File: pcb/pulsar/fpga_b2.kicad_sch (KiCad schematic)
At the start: 85 parts

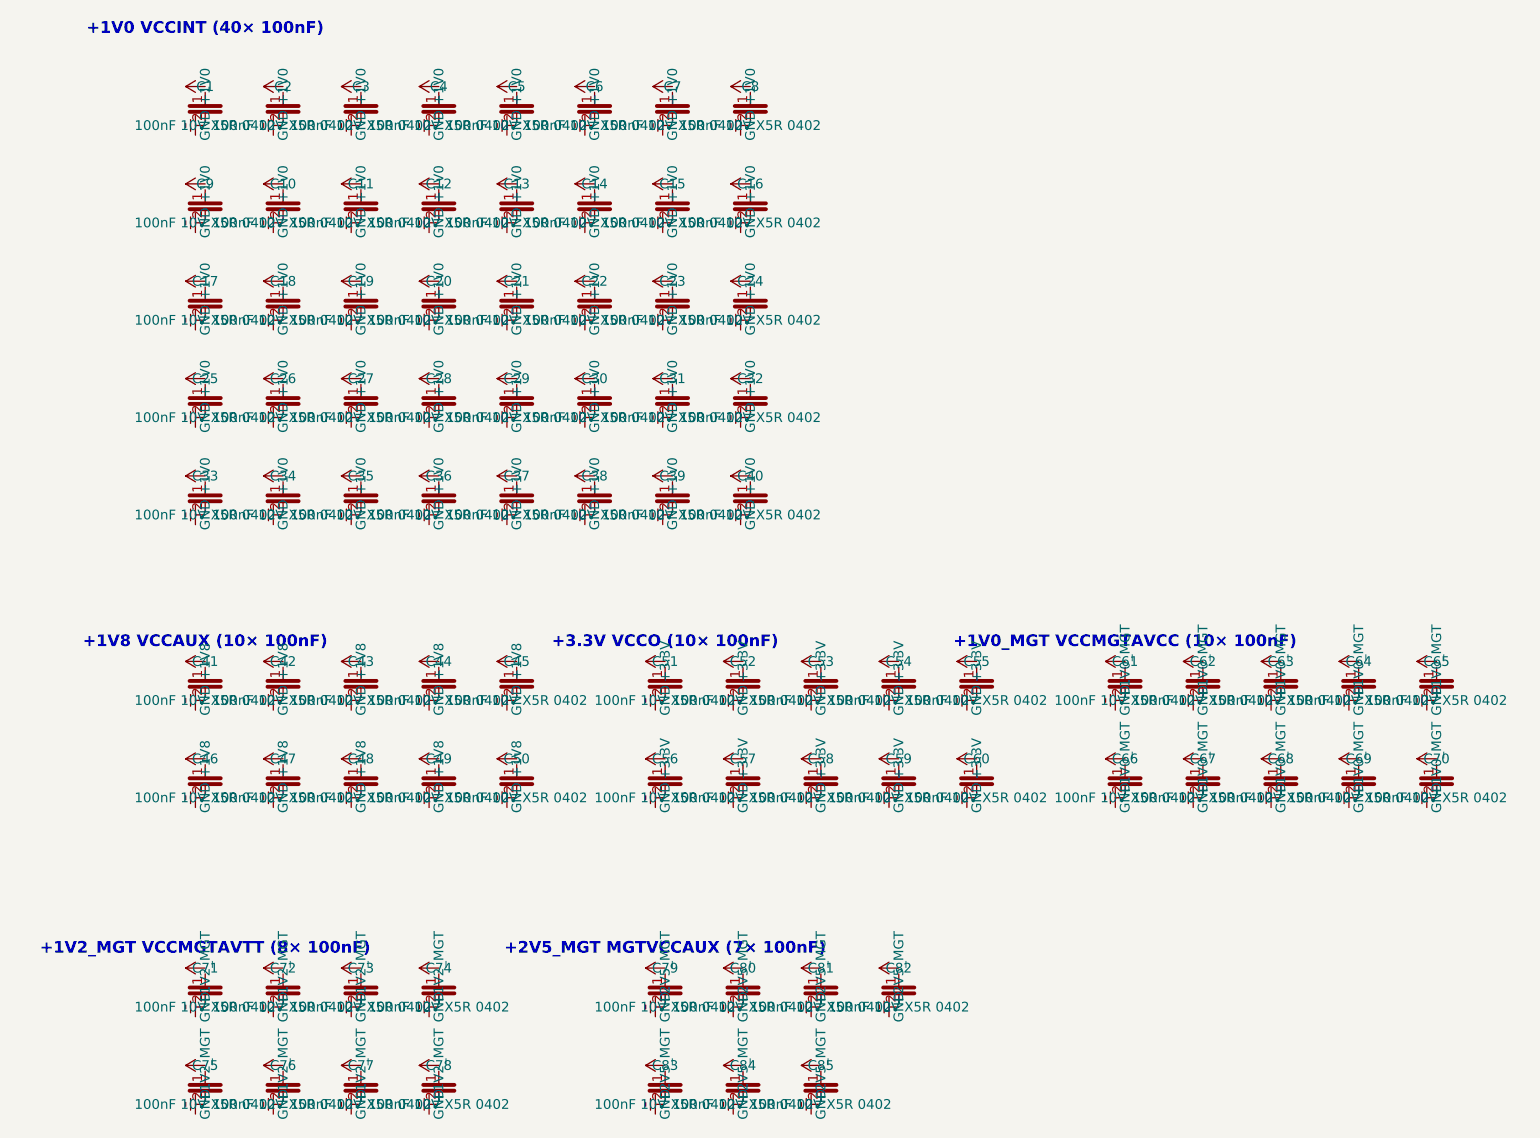
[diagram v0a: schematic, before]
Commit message: feat: let everything to route
Signed-off-by: Axel Ibarrondo <135344010+Axel84727@users.noreply.github.com>
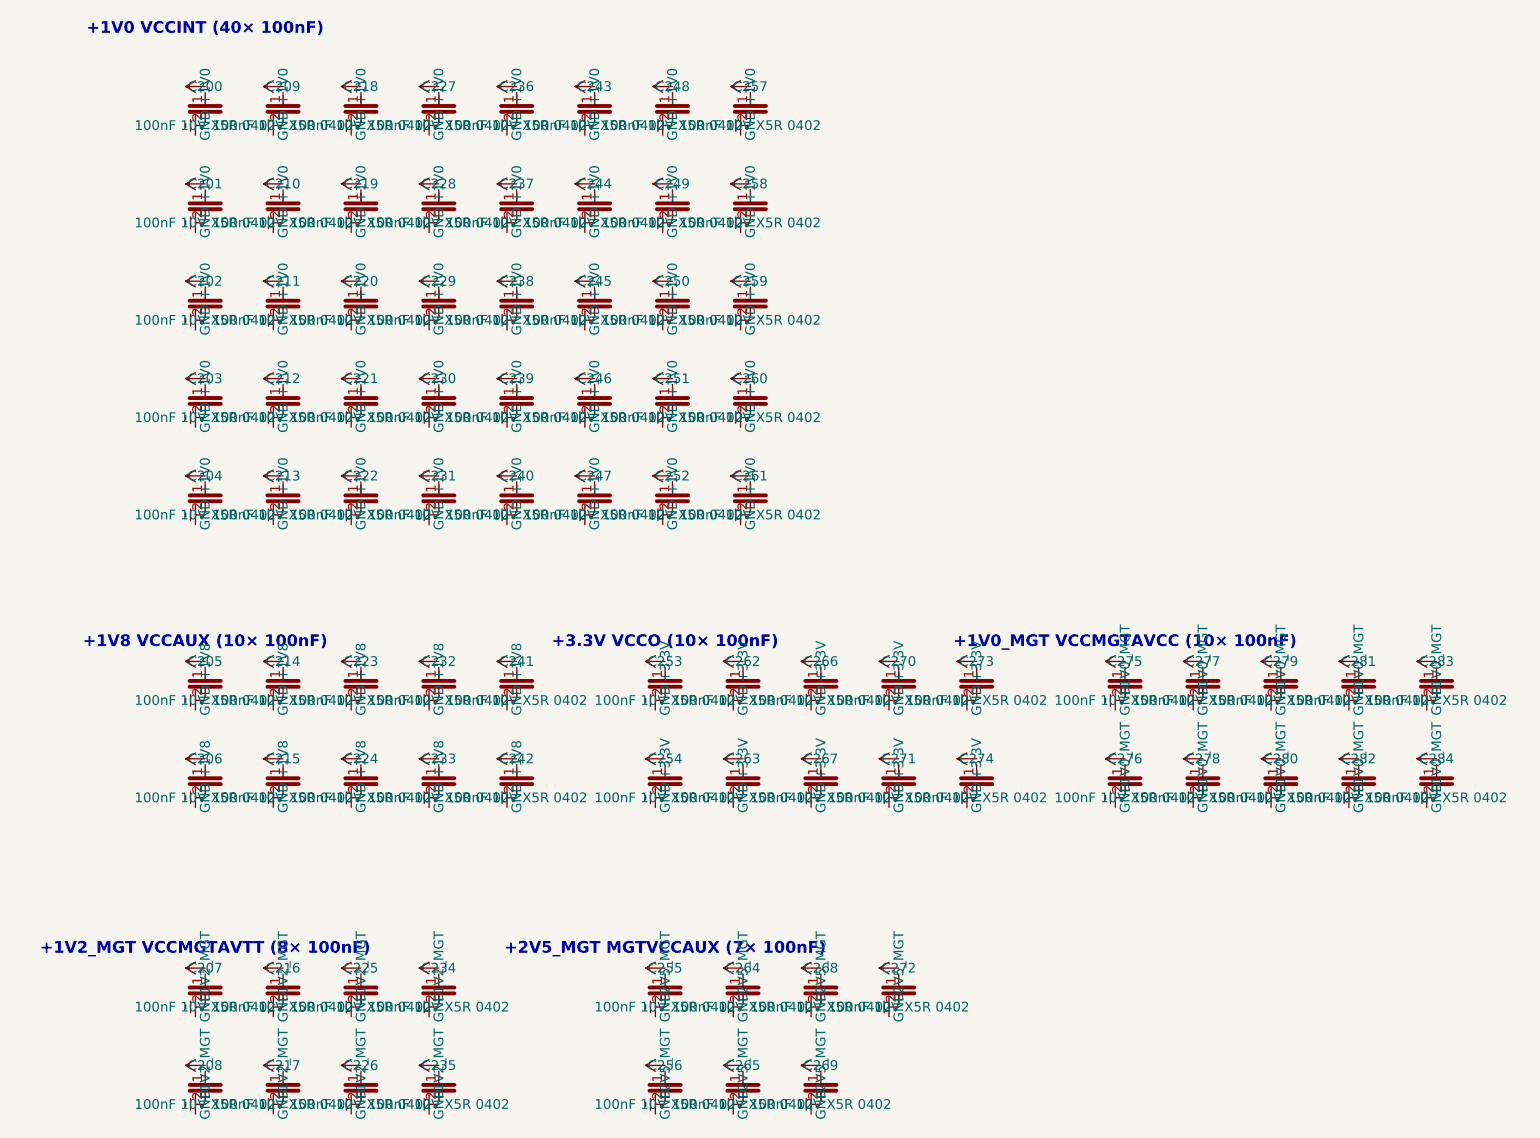
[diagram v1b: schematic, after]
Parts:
- renumbered C1 to C200, C9 to C201, C17 to C202, C25 to C203, C33 to C204, C41 to C205, C46 to C206, C71 to C207, C75 to C208, C2 to C209, C10 to C210, C18 to C211, C26 to C212, C34 to C213, C42 to C214, C47 to C215, C72 to C216, C76 to C217, C3 to C218, C11 to C219, C19 to C220, C27 to C221, C35 to C222, C43 to C223, C48 to C224, C73 to C225, C77 to C226, C4 to C227, C12 to C228, C20 to C229, C28 to C230, C36 to C231, C44 to C232, C49 to C233, C74 to C234, C78 to C235, C5 to C236, C13 to C237, C21 to C238, C29 to C239, C37 to C240, C45 to C241, C50 to C242, C6 to C243, C14 to C244, C22 to C245, C30 to C246, C38 to C247, C7 to C248, C15 to C249, C23 to C250, C31 to C251, C39 to C252, C51 to C253, C56 to C254, C79 to C255, C83 to C256, C8 to C257, C16 to C258, C24 to C259, C32 to C260, C40 to C261, C52 to C262, C57 to C263, C80 to C264, C84 to C265, C53 to C266, C58 to C267, C81 to C268, C85 to C269, C54 to C270, C59 to C271, C82 to C272, C55 to C273, C60 to C274, C61 to C275, C66 to C276, C62 to C277, C67 to C278, C63 to C279, C68 to C280, C64 to C281, C69 to C282, C65 to C283, C70 to C284
